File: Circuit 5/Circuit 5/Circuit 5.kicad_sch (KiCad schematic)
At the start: 34 parts, among them SW1 RIGHT, SW2 LEFT, SW3 Load, SW4 SW_DIP_x04, U1 74LS14, U13 74LS08, U14 74LS08, U15 74LS08, U16 74LS32, U2 74LS32, U3 74LS32, U4 74LS194, U7 74LS04, U8 74LS32

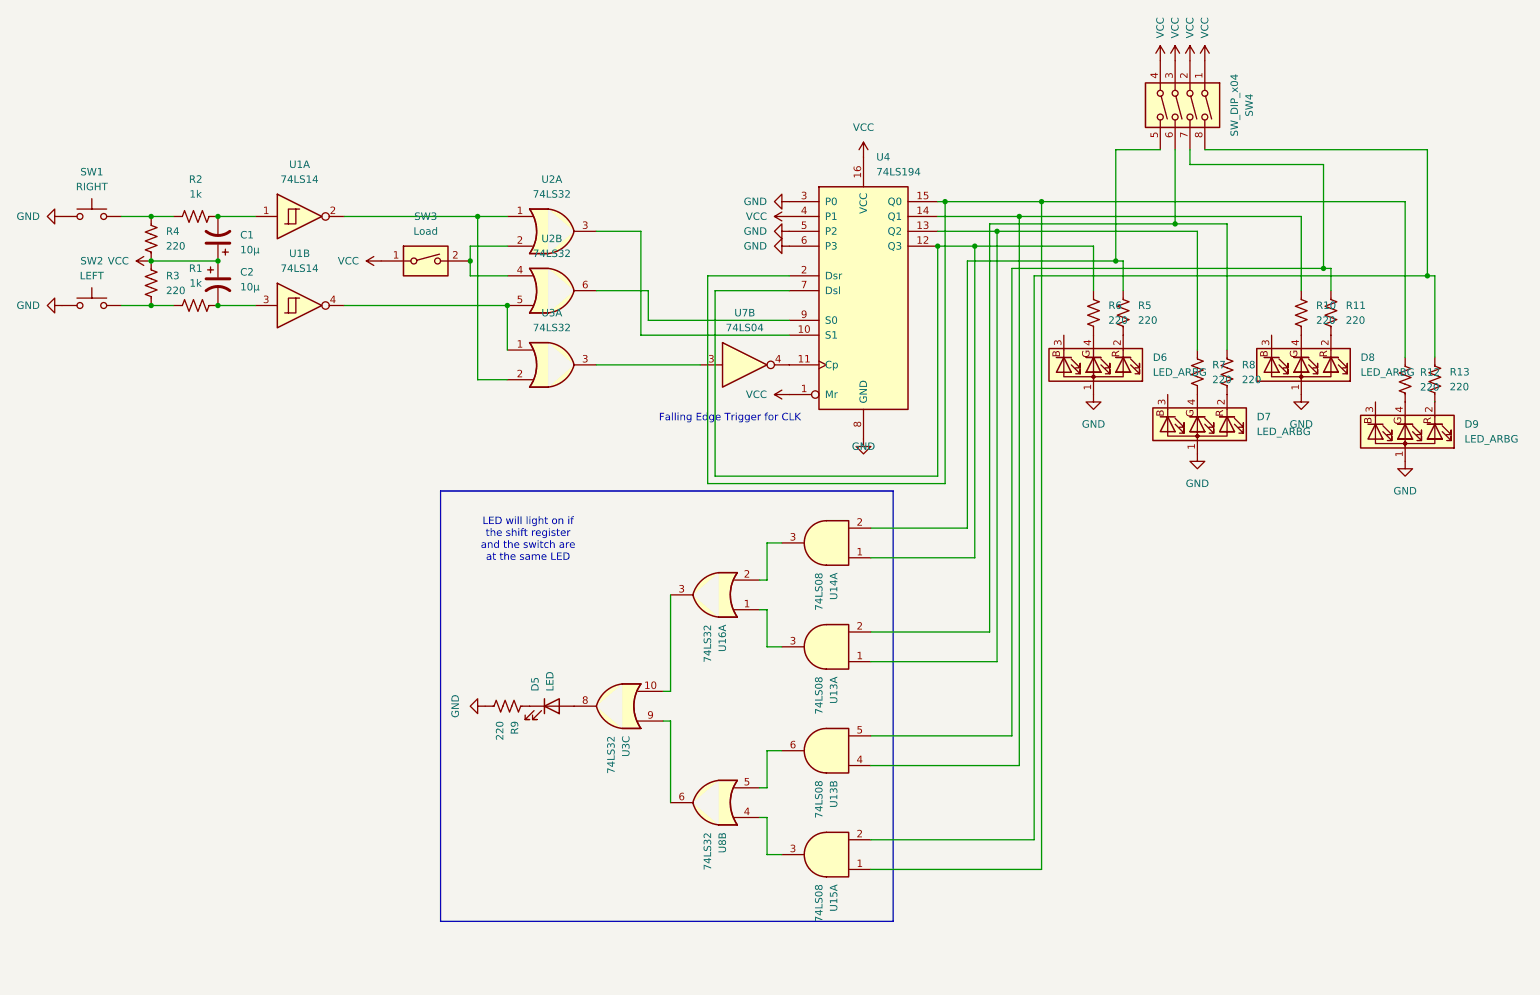
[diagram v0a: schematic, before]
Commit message: Add files via upload
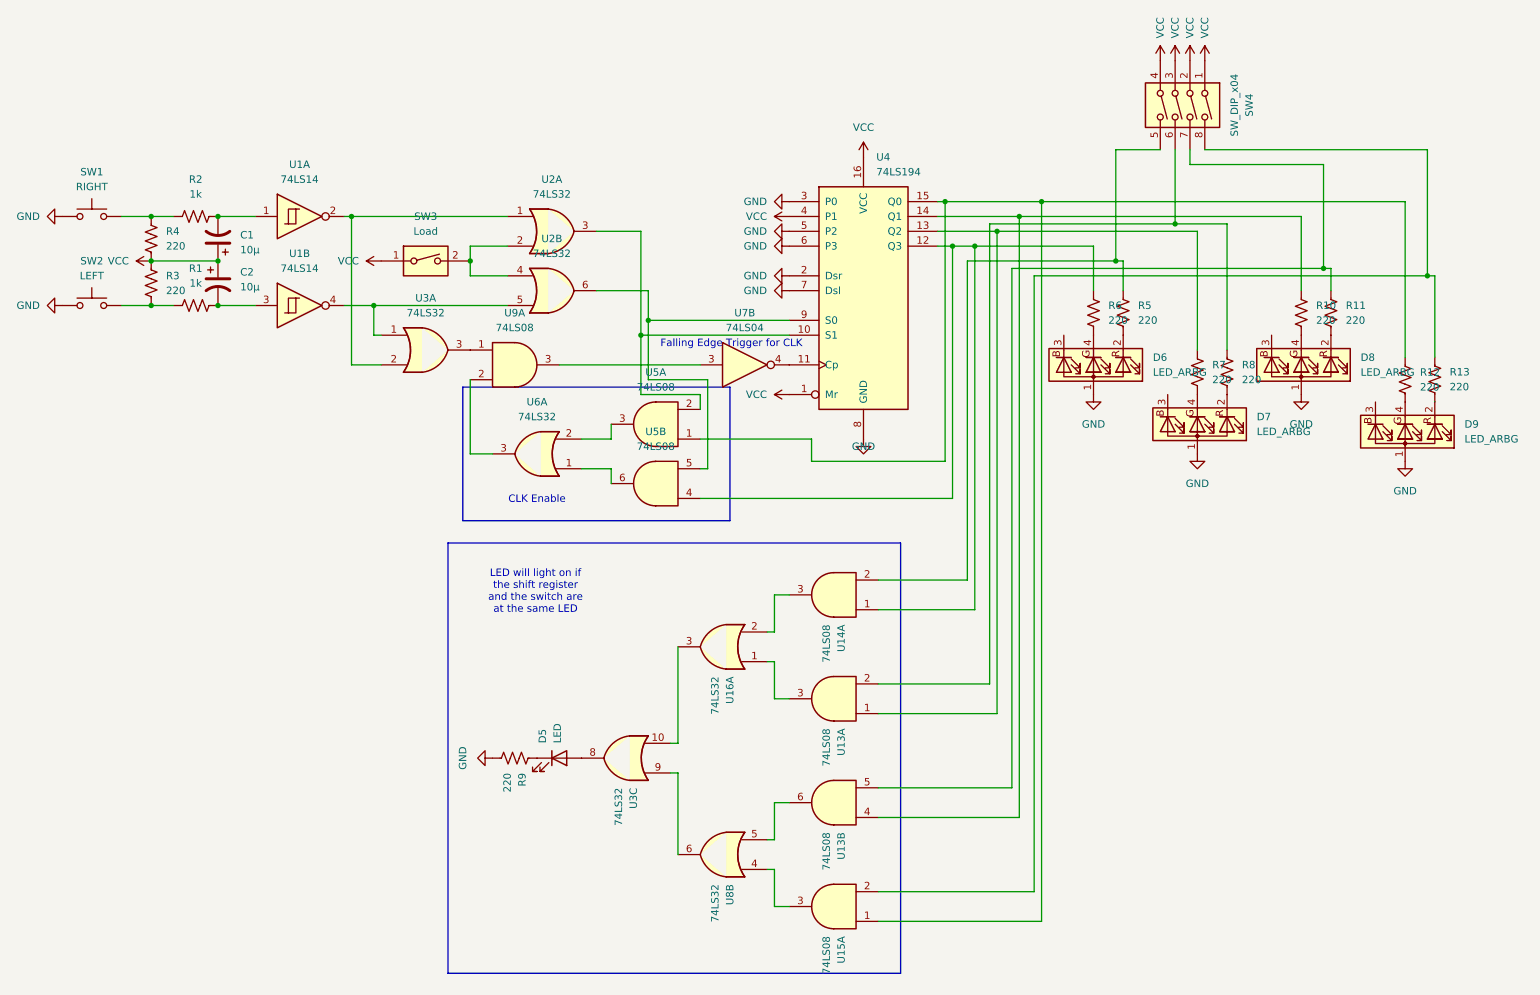
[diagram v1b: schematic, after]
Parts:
- added U5, U9: 74LS08, symbol 74xx:74LS08
- added U6: 74LS32, symbol 74xx:74LS32
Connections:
- net GND: now also U4.2 (Dsr), U4.7 (Dsl)
- net at R12.1, U15.1, U4.15 (Q0): now also U5.1; no longer U4.2 (Dsr)
- net at U7.3: now also U9.3; no longer U3.3
- net at U2.3, U4.10 (S1): now also U5.2
- net at R6.1, U14.1, U4.12 (Q3): now also U5.4; no longer U4.7 (Dsl)
- net at U2.6, U4.9 (S0): now also U5.5
- new net: U5.6, U6.1
- new net: U5.3, U6.2
- new net: U3.3, U9.1
- new net: U6.3, U9.2
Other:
- note added: "CLK Enable"
- moved on the sheet: D5, R9, U13A, U13B, U14A, U15A, U16A, U3A, U3C, U8B
